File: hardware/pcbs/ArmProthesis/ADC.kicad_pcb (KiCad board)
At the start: 4 copper layers, 56.7 x 50.8 mm, 27 parts, among them J1 H_16_2.54mm, SW1 SW_Reed_SPDT, SW2 SW_Reed_SPDT, SW3 SW_Reed_SPDT, U1 AD7606BSTZ

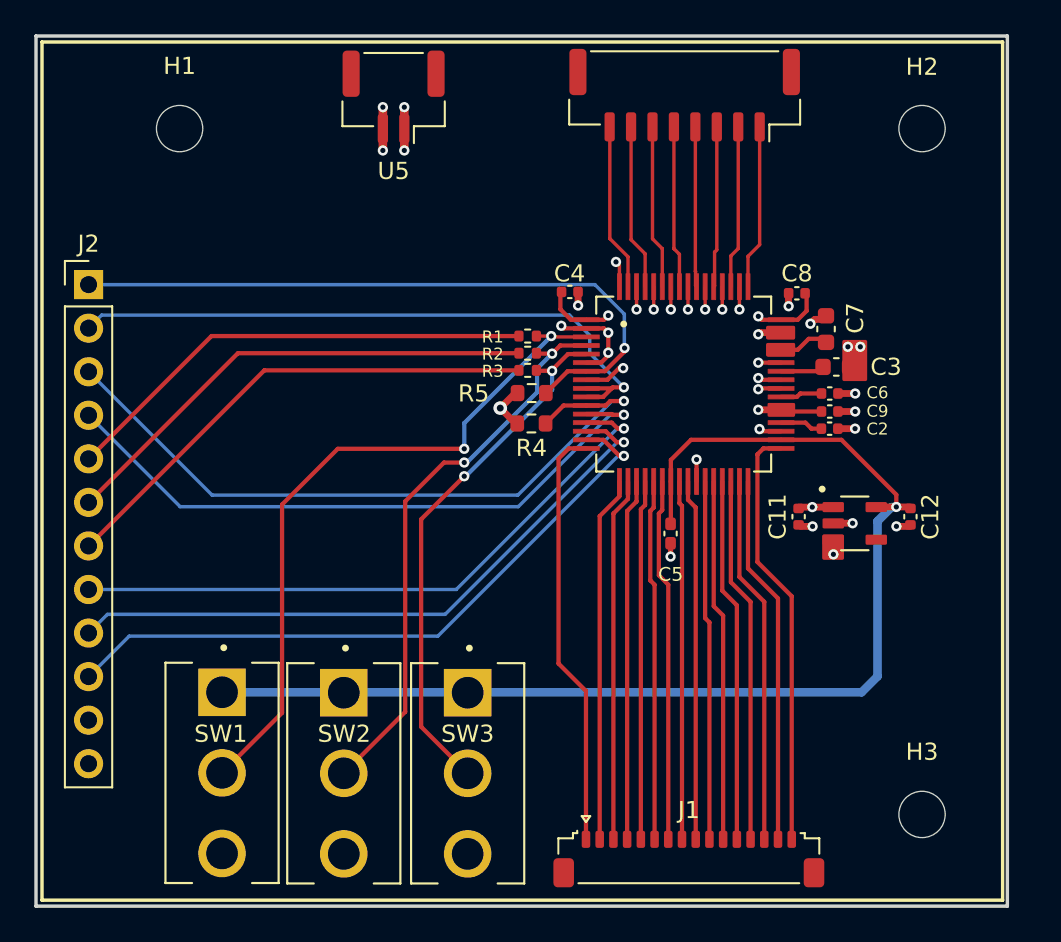
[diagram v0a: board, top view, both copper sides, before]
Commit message: Ordered versions
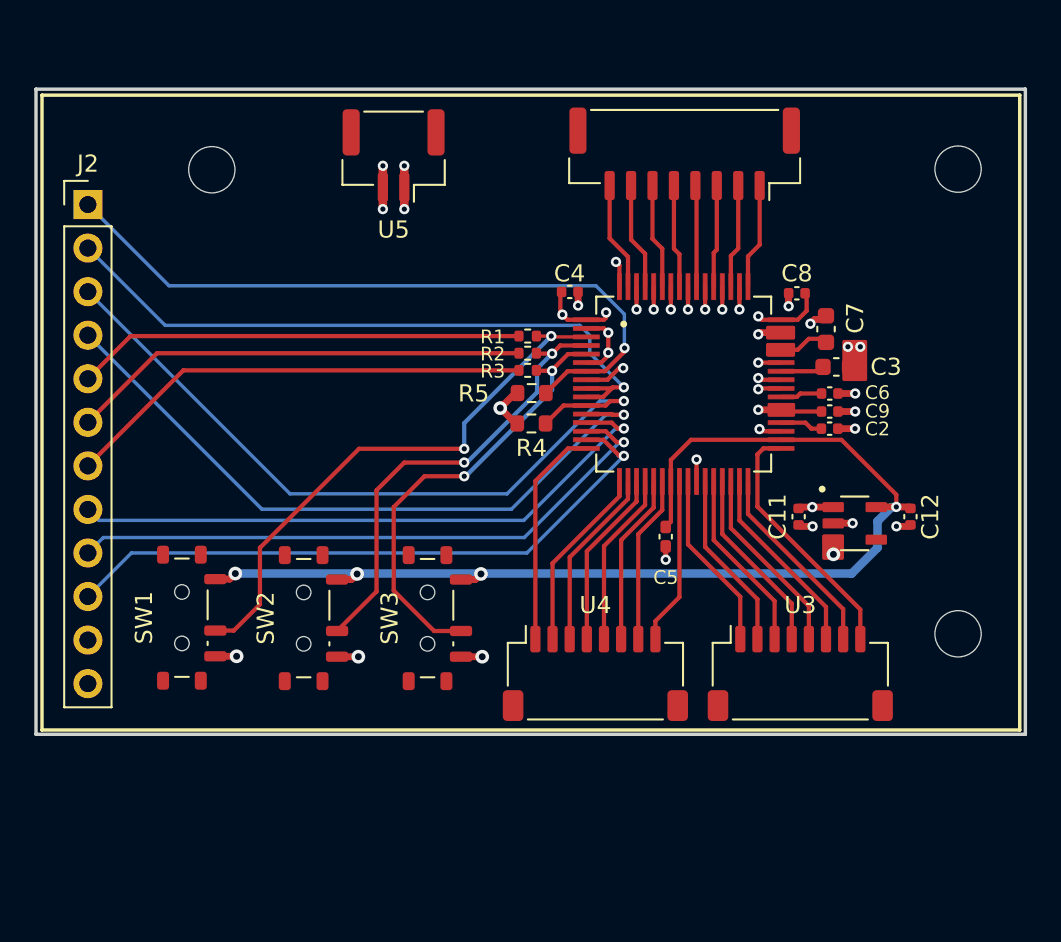
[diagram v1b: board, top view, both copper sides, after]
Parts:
- removed J1: H_16_2.54mm, Connector_JST:JST_SUR_SM16B-SURS-TF_1x16-1MP_P0.80mm_Horizontal
- added U3: ~, Connector_JST:JST_SH_SM08B-SRSS-TB_1x08-1MP_P1.00mm_Horizontal, F.Cu at (183.7, 101.8)
- added U4: ~, Connector_JST:JST_SH_SM08B-SRSS-TB_1x08-1MP_P1.00mm_Horizontal, F.Cu at (171.8, 101.8)
- SW1, SW2, SW3: footprint Switches:switch1 -> Button_Switch_SMD:SW_SPDT_Shouhan_MSK12C02
- moved H3 10.7 mm to (192.9, 99.5)
- moved SW1 9.35 mm to (147.6, 98.5)
- moved SW3 9.35 mm to (162.0, 98.5)
- moved SW2 9.35 mm to (154.7, 98.5)
- moved J2 4.67 mm to (142.2, 74.4)
- moved U2 3.42 mm to (177.0, 71.5)
- moved U5 3.42 mm to (160.0, 71.6)
- moved H2 3.16 mm to (192.9, 72.4)
- moved H1 3.05 mm to (149.4, 72.4)
- moved C5 0.34 mm to (175.8, 93.8)
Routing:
- net DB0: track 24.7 -> 13.0 mm
- net DB6: track 21.2 -> 9.77 mm
- net DB7/DOUTA: track 20.9 -> 9.77 mm
- net DB5: track 21.1 -> 9.98 mm
- net DB4: track 21.0 -> 10.2 mm
- net DB3: track 21.1 -> 10.4 mm
- net DB2: track 21.2 -> 10.6 mm
- net DB8DOUTB: track 21.1 -> 10.5 mm
- net DB1: track 21.3 -> 10.8 mm
- net DB9: track 21.0 -> 10.5 mm
- net DB10: track 21.1 -> 10.7 mm
- net DB11: track 21.2 -> 10.9 mm
- net DB12: track 21.3 -> 11.1 mm
- net DB13: track 21.5 -> 11.3 mm
- net DB14: track 21.6 -> 11.5 mm
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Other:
- board size 56.7 x 50.8 mm -> 57.7 x 37.6 mm
